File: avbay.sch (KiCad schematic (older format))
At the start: 16 parts, among them P1 CONN_2, P2 CONN_6, P3 CONN_2, P4 CONN_2, P6 CONN_01X12, SW2 SW_PUSH, SW3 SW_PUSH

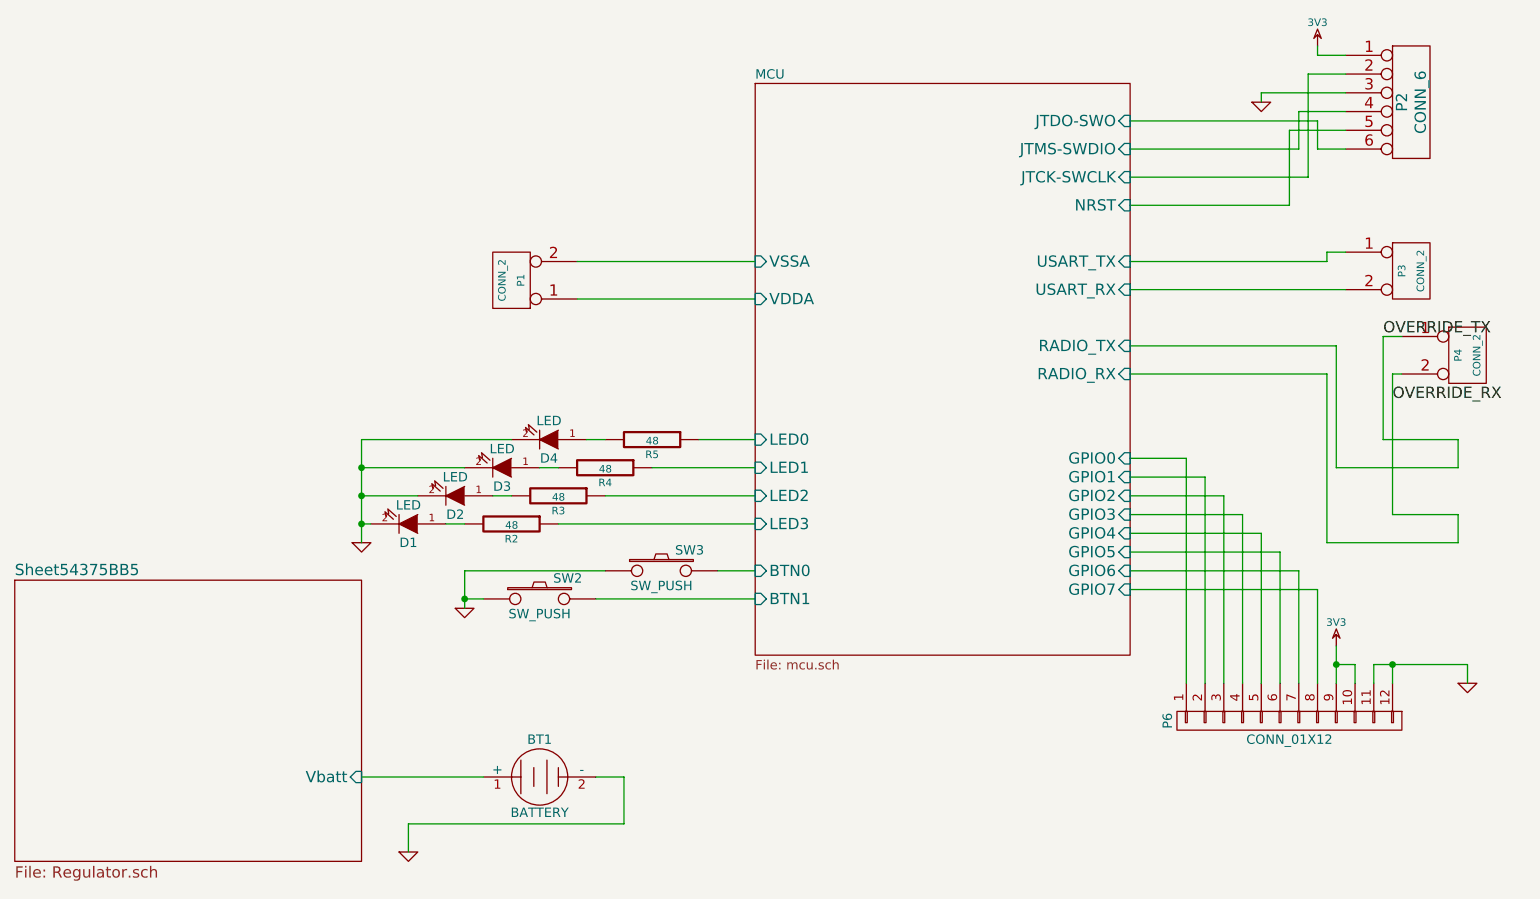
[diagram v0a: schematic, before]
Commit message: Made breakout board
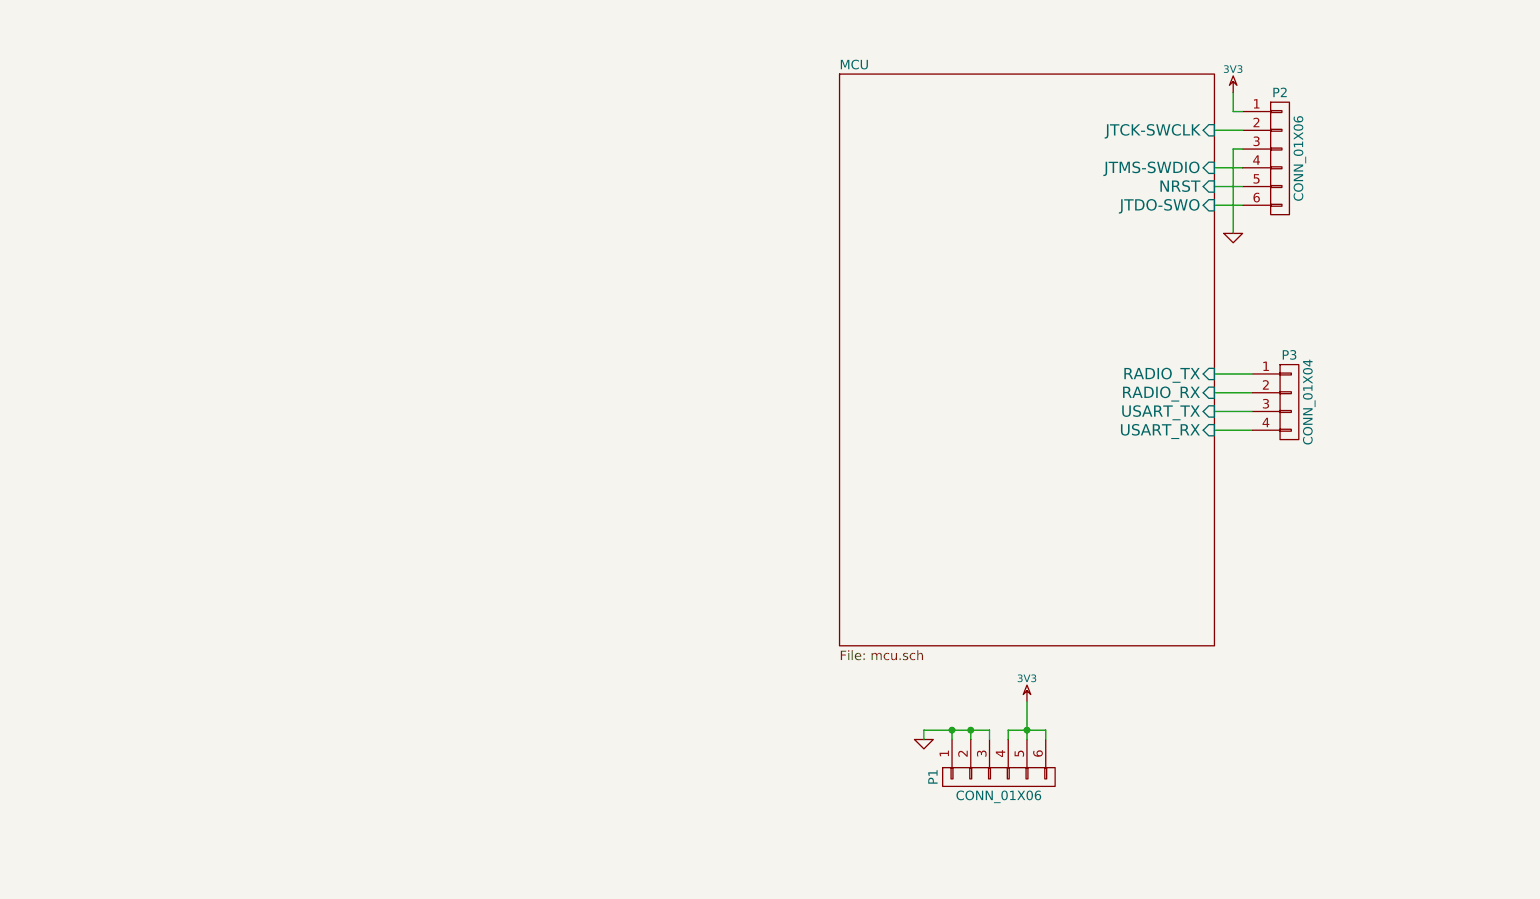
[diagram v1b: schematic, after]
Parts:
- removed BT1: BATTERY, ~, symbol BATTERY
- removed D1, D2, D3, D4: LED, symbol LED
- removed P1, P3, P4: CONN_2, symbol CONN_2
- removed P2: CONN_6, symbol CONN_6
- removed P6: CONN_01X12, symbol CONN_01X12
- removed R2, R3, R4, R5: 48, symbol R
- removed SW2, SW3: SW_PUSH, symbol SW_PUSH
- added P1, P2: CONN_01X06, Pin_Headers:Pin_Header_Straight_1x06, symbol CONN_01X06
- added P3: CONN_01X04, Pin_Headers:Pin_Header_Straight_1x04, symbol CONN_01X04
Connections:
- net 3V3: now also P1.4 (P4), P1.5 (P5), P1.6 (P6), P2.1 (P1)
- net GND: now also P1.1 (P1), P1.2 (P2), P1.3 (P3), P2.3 (P3)
- net MCU/JTCK-SWCLK: now also P2.2 (P2)
- net MCU/JTDO-SWO: now also P2.6 (P6)
- net MCU/JTMS-SWDIO: now also P2.4 (P4)
- net MCU/NRST: now also P2.5 (P5)
- net MCU/USART_RX: now also P3.4 (P4)
- net MCU/USART_TX: now also P3.3 (P3)
- new net MCU/RADIO_RX: P3.2 (P2)
- new net MCU/RADIO_TX: P3.1 (P1)
